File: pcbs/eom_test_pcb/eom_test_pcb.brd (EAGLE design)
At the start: 160 x 48 mm, 72 parts

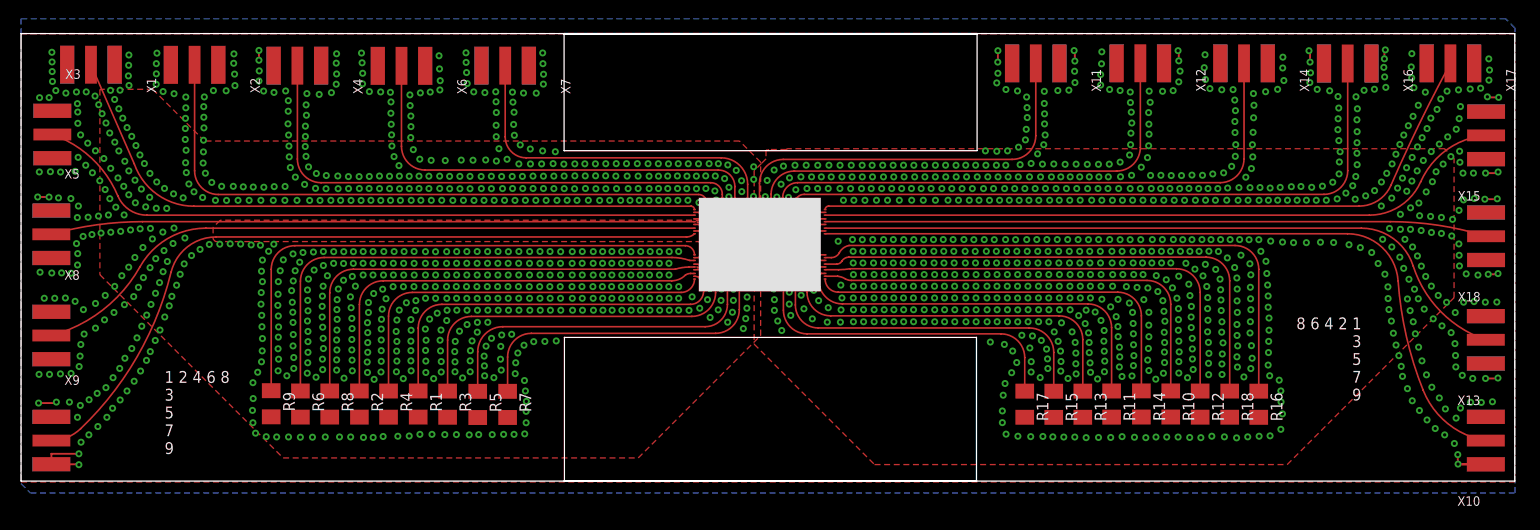
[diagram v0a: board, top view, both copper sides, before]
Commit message: Push after sending to PCBWay in this state
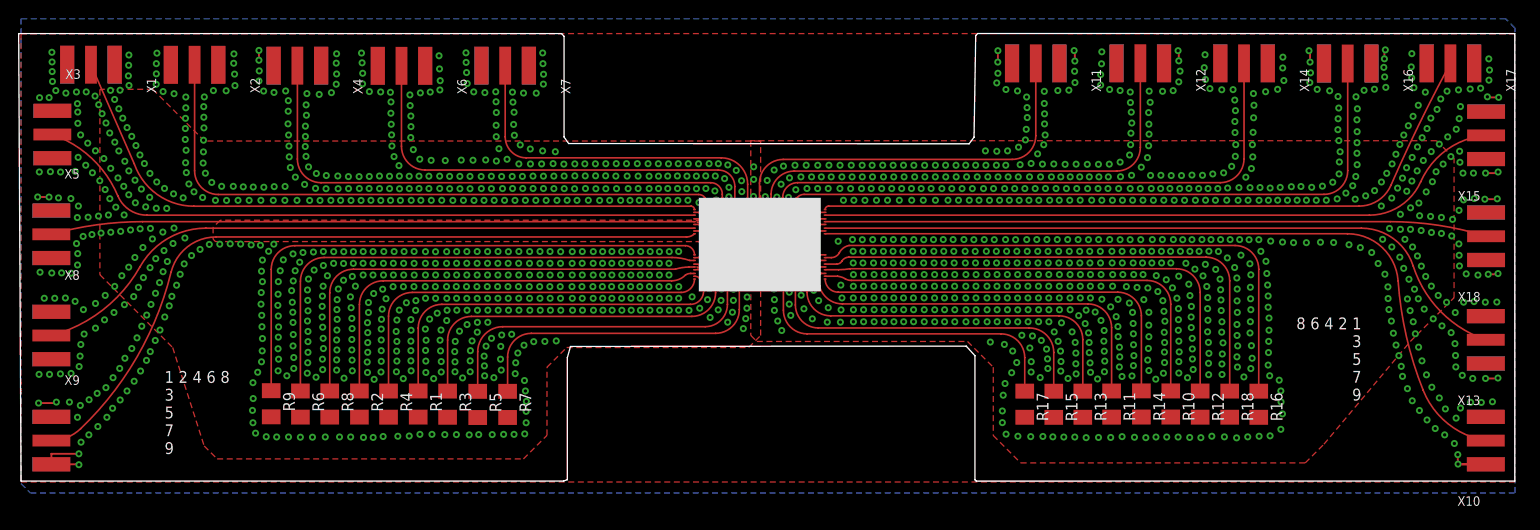
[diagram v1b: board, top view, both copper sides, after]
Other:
- board size 160 x 48 mm -> 160.3 x 47.9 mm
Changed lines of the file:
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@@
 <setting verticaltext="up"/>
 </settings>
-<grid distance="100" unitdist="mil" unit="mil" style="lines" multiple="1" display="no" altdistance="0.001" altunitdist="mil" altunit="mil"/>
+<grid distance="10" unitdist="mil" unit="mil" style="lines" multiple="1" display="no" altdistance="0.001" altunitdist="mil" altunit="mil"/>
 <layers>
 <layer number="1" name="Top" color="4" fill="1" visible="yes" active="yes"/>
@@
 <board>
 <plain>
-<wire x1="0" y1="52.07" x2="160" y2="52.07" width="0" layer="20"/>
+<wire x1="0" y1="52.07" x2="58.109459375" y2="52.07" width="0" layer="20"/>
+<wire x1="58.109459375" y1="52.07" x2="58.5160625" y2="52.22263125" width="0" layer="20"/>
+<wire x1="58.5160625" y1="52.22263125" x2="58.5166" y2="65.291534375" width="0" layer="20"/>
+<wire x1="58.5166" y1="65.291534375" x2="58.8541125" y2="66.4930875" width="0" layer="20"/>
+<wire x1="58.8541125" y1="66.4930875" x2="101.2459" y2="66.52275" width="0" layer="20"/>
+<wire x1="101.2459" y1="66.52275" x2="102.17505625" y2="65.502840625" width="0" layer="20"/>
+<wire x1="102.17505625" y1="65.502840625" x2="102.17505625" y2="52.21094375" width="0" layer="20"/>
+<wire x1="102.17505625" y1="52.21094375" x2="102.320903125" y2="52.065096875" width="0" layer="20"/>
+<wire x1="102.320903125" y1="52.065096875" x2="160" y2="52.07" width="0" layer="20"/>
 <wire x1="160" y1="52.07" x2="160" y2="100" width="0" layer="20"/>
-<wire x1="160" y1="100" x2="0" y2="100" width="0" layer="20"/>
-<wire x1="0" y1="100" x2="0" y2="52.07" width="0" layer="20"/>
+<wire x1="160" y1="100" x2="102.4691875" y2="100.0101875" width="0" layer="20"/>
+<wire x1="102.4691875" y1="100.0101875" x2="102.261415625" y2="99.802415625" width="0" layer="20"/>
+<wire x1="102.261415625" y1="99.802415625" x2="102.07911875" y2="88.90134375" width="0" layer="20"/>
+<wire x1="102.07911875" y1="88.90134375" x2="101.551584375" y2="88.197640625" width="0" layer="20"/>
+<wire x1="101.551584375" y1="88.197640625" x2="58.65636875" y2="88.223196875" width="0" layer="20"/>
+<wire x1="58.65636875" y1="88.223196875" x2="58.1612" y2="88.9323375" width="0" layer="20"/>
+<wire x1="58.1612" y1="88.9323375" x2="58.167496875" y2="99.7101125" width="0" layer="20"/>
+<wire x1="58.167496875" y1="99.7101125" x2="57.90395" y2="100" width="0" layer="20"/>
+<wire x1="57.90395" y1="100" x2="-0.254" y2="100" width="0" layer="20"/>
+<wire x1="-0.254" y1="100" x2="0" y2="52.07" width="0" layer="20"/>
 <rectangle x1="72.59" y1="72.39" x2="85.671" y2="82.423" layer="21"/>
-<dimension x1="72.39" y1="82.423" x2="72.39" y2="81.153" x3="70.8406" y3="81.788" textsize="0.254" layer="25" width="0.0254" unit="mil" precision="0"/>
-<dimension x1="72.39" y1="82.423" x2="72.39" y2="81.153" x3="69.85" y3="81.788" textsize="0.254" layer="25" width="0.0254" unit="mic" precision="0"/>
-<dimension x1="85.671" y1="82.423" x2="85.67" y2="81.153" x3="87.122196875" y3="81.78685625" textsize="0.254" layer="25" width="0.0254" unit="mil" precision="1"/>
-<dimension x1="85.671" y1="82.423" x2="86.1314" y2="82.423" x3="85.9012" y3="81.153" textsize="0.254" layer="25" width="0.0254" unit="mil" precision="1"/>
-<rectangle x1="58.17" y1="87.46" x2="102.4" y2="99.99" layer="46"/>
-<rectangle x1="58.2" y1="52.06" x2="102.34" y2="67.46" layer="46"/>
-<rectangle x1="58.17" y1="99.99" x2="102.4" y2="100.01" layer="46"/>
 <rectangle x1="71.597775" y1="72.45223125" x2="72.58964375" y2="82.3572125" layer="29"/>
 <rectangle x1="85.68486875" y1="72.4573125" x2="86.6767375" y2="82.36229375" layer="29"/>
@@
             7
             9</text>
+<rectangle x1="70.538034375" y1="72.451975" x2="71.597821875" y2="82.35688125" layer="29"/>
+<rectangle x1="86.676075" y1="72.457234375" x2="87.7358625" y2="82.362140625" layer="29"/>
 </plain>
 <attributes>
@@
 <param name="mdViaViaSameLayer" value="6mil"/>
 <param name="mnLayersViaInSmd" value="2"/>
-<param name="mdCopperDimension" value="40mil"/>
+<param name="mdCopperDimension" value="30mil"/>
 <param name="mdDrill" value="6mil"/>
 <param name="mdSmdStop" value="0mil"/>
@@
 <vertex x="8.448040625" y="94.015559375"/>
 <vertex x="8.448040625" y="74.170540625"/>
-<vertex x="28.069540625" y="54.549040625"/>
-<vertex x="66.11111875" y="54.549040625"/>
+<vertex x="16.24208125" y="66.3765"/>
+<vertex x="19.61515" y="55.833009375"/>
+<vertex x="21.004478125" y="54.44368125"/>
+<vertex x="53.8115" y="54.44368125"/>
+<vertex x="56.332703125" y="56.964884375"/>
+<vertex x="56.332703125" y="64.26408125"/>
+<vertex x="58.445121875" y="66.3765"/>
+<vertex x="77.938578125" y="66.3765"/>
 <vertex x="79.220059375" y="67.65798125"/>
-<vertex x="79.220059375" y="86.233"/>
-<vertex x="76.959459375" y="88.4936"/>
+<vertex x="79.220059375" y="88.4936"/>
 <vertex x="19.65198125" y="88.4936"/>
 <vertex x="14.112240625" y="94.033340625"/>
@@
 <via x="108.8898" y="87.11691875" extent="1-16" drill="0.35" diameter="0.55"/>
 <polygon width="0.0762" layer="1" spacing="0.254" isolate="0.1524" orphans="yes" thermals="no">
-<vertex x="79.796640625" y="87.5157"/>
-<vertex x="79.796640625" y="86.580978125"/>
-<vertex x="79.31658125" y="86.10091875"/>
-<vertex x="78.5241" y="85.3084375"/>
-<vertex x="78.5241" y="66.735959375"/>
-<vertex x="91.42221875" y="53.837840625"/>
-<vertex x="104.764840625" y="53.837840625"/>
-<vertex x="135.625840625" y="53.837840625"/>
+<vertex x="78.1661625" y="88.524790625"/>
+<vertex x="78.1661625" y="67.67205"/>
+<vertex x="78.812946875" y="67.025265625"/>
+<vertex x="101.382553125" y="67.025265625"/>
+<vertex x="104.14" y="64.26781875"/>
+<vertex x="104.14" y="56.95124375"/>
+<vertex x="107.074765625" y="54.016478125"/>
+<vertex x="137.55893125" y="54.016478125"/>
+<vertex x="139.5595375" y="56.017084375"/>
+<vertex x="148.813265625" y="67.025265625"/>
 <vertex x="153.49728125" y="71.70928125"/>
 <vertex x="153.49728125" y="86.657178125"/>
-<vertex x="152.486359375" y="87.6681"/>
-<vertex x="82.0674" y="87.6681"/>
-<vertex x="81.98358125" y="87.58428125"/>
-<vertex x="80.1116" y="87.58428125"/>
-<vertex x="80.058259375" y="87.530940625"/>
-<vertex x="79.91348125" y="87.530940625"/>
-<vertex x="79.905859375" y="87.52331875"/>
-<vertex x="79.80171875" y="87.52331875"/>
-<vertex x="79.796640625" y="87.518240625"/>
+<vertex x="151.62966875" y="88.524790625"/>
 </polygon>
 <via x="110.096046875" y="69.134225" extent="1-16" drill="0.35" diameter="0.55"/>
